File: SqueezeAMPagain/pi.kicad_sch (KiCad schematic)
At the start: 4 parts, among them J4 Raspberry_Pi_2_3

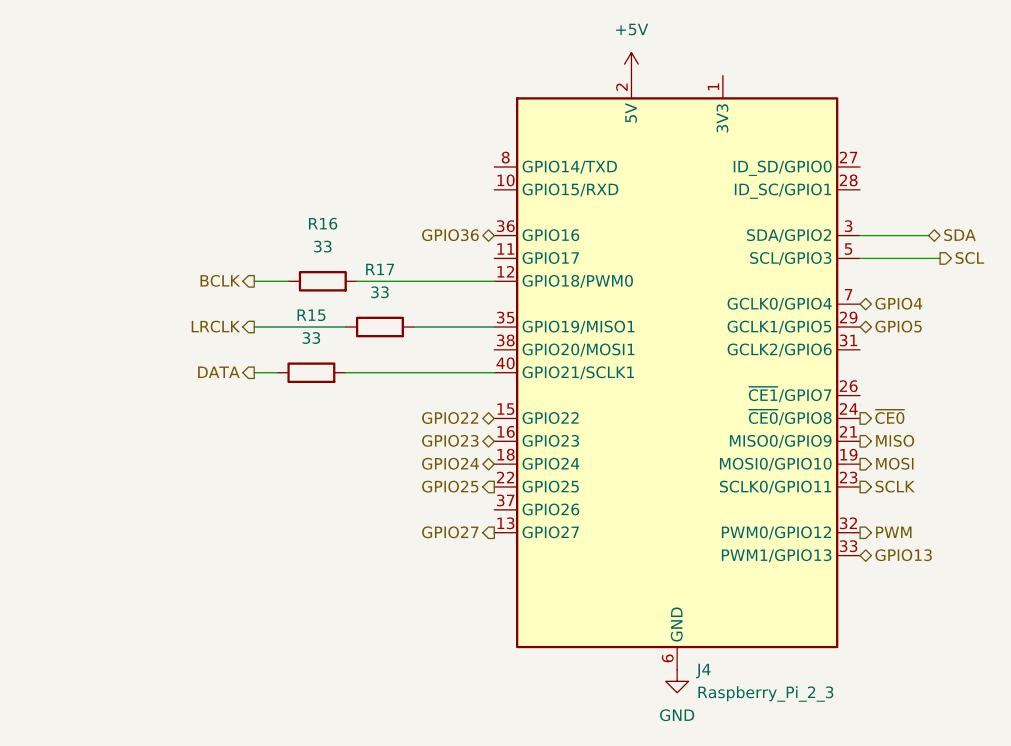
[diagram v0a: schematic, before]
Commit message: Update SqueezeAMPagain.kicad_pcb, SqueezeAMPagain.kicad_prl, SqueezeAMPagain.kicad_pro, and 7 more files
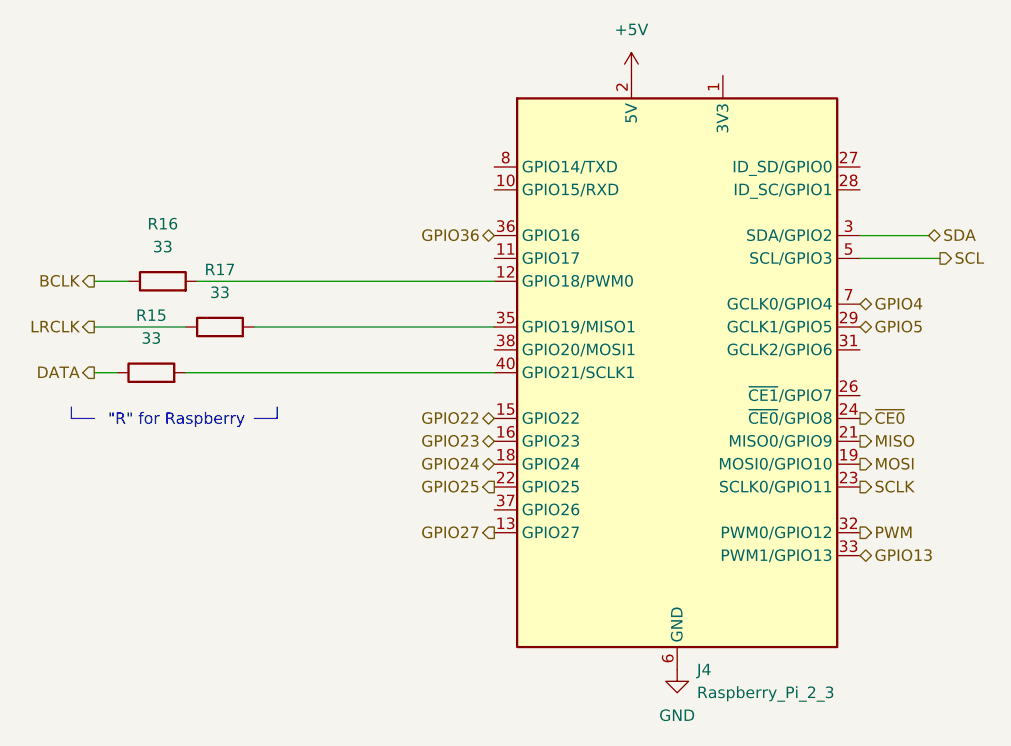
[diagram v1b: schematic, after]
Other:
- note added: ""R" for Raspberry"
- moved on the sheet: R15, R16, R17
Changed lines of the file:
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@@
 	(generator_version "8.0")
 	(paper "A4")
+	(polyline
+		(pts
+			(xy 19.05 91.44) (xy 19.05 92.71)
+		)
+		(stroke
+			(width 0)
+			(type default)
+		)
+	)
+	(polyline
+		(pts
+			(xy 41.91 91.44) (xy 41.91 92.71)
+		)
+		(stroke
+			(width 0)
+			(type default)
+		)
+	)
 	(wire
 		(pts
-			(xy 50.8 77.47) (xy 66.04 77.47)
+			(xy 33.02 77.47) (xy 66.04 77.47)
 		)
 		(stroke
@@
 		)
 	)
+	(polyline
+		(pts
+			(xy 39.37 92.71) (xy 41.91 92.71)
+		)
+		(stroke
+			(width 0)
+			(type default)
+		)
+	)
 	(wire
 		(pts
-			(xy 39.37 77.47) (xy 43.18 77.47)
+			(xy 21.59 77.47) (xy 25.4 77.47)
 		)
 		(stroke
@@
 	(wire
 		(pts
-			(xy 39.37 82.55) (xy 49.53 82.55)
+			(xy 21.59 82.55) (xy 31.75 82.55)
+		)
+		(stroke
+			(width 0)
+			(type default)
+		)
+	)
+	(polyline
+		(pts
+			(xy 19.05 92.71) (xy 21.59 92.71)
 		)
 		(stroke
@@
 	(wire
 		(pts
-			(xy 57.15 82.55) (xy 66.04 82.55)
+			(xy 39.37 82.55) (xy 66.04 82.55)
 		)
 		(stroke
@@
 	(wire
 		(pts
-			(xy 39.37 87.63) (xy 41.91 87.63)
+			(xy 21.59 87.63) (xy 24.13 87.63)
 		)
 		(stroke
@@
 	(wire
 		(pts
-			(xy 49.53 87.63) (xy 66.04 87.63)
-		)
-		(stroke
-			(width 0)
-			(type default)
+			(xy 31.75 87.63) (xy 66.04 87.63)
+		)
+		(stroke
+			(width 0)
+			(type default)
+		)
+	)
+	(text "\"R\" for Raspberry"
+		(exclude_from_sim no)
+		(at 30.734 92.964 0)
+		(effects
+			(font
+				(size 1.27 1.27)
+			)
 		)
 	)
@@
 	(hierarchical_label "LRCLK"
 		(shape output)
-		(at 39.37 82.55 180)
+		(at 21.59 82.55 180)
 		(fields_autoplaced yes)
 		(effects
@@
 	(hierarchical_label "DATA"
 		(shape output)
-		(at 39.37 87.63 180)
+		(at 21.59 87.63 180)
 		(fields_autoplaced yes)
 		(effects
@@
 	(hierarchical_label "BCLK"
 		(shape output)
-		(at 39.37 77.47 180)
+		(at 21.59 77.47 180)
 		(fields_autoplaced yes)
 		(effects
@@
 	(symbol
 		(lib_id "Device:R")
-		(at 45.72 87.63 90)
+		(at 27.94 87.63 90)
 		(unit 1)
 		(exclude_from_sim no)
@@
 		(fields_autoplaced yes)
 		(property "Reference" "R15"
-			(at 45.72 81.28 90)
+			(at 27.94 81.28 90)
 			(effects
 				(font
@@
 		)
 		(property "Value" "33"
-			(at 45.72 83.82 90)
+			(at 27.94 83.82 90)
 			(effects
 				(font
@@
 		)
 		(property "Footprint" "Resistor_SMD:R_0402_1005Metric"
-			(at 45.72 89.408 90)
+			(at 27.94 89.408 90)
 			(effects
 				(font
@@
 		)
 		(property "Datasheet" "~"
-			(at 45.72 87.63 0)
+			(at 27.94 87.63 0)
 			(effects
 				(font
@@
 		)
 		(property "Description" "Resistor"
-			(at 45.72 87.63 0)
+			(at 27.94 87.63 0)
 			(effects
 				(font
@@
 	(symbol
 		(lib_id "Device:R")
-		(at 46.99 77.47 90)
+		(at 29.21 77.47 90)
 		(unit 1)
 		(exclude_from_sim no)
@@
 		(fields_autoplaced yes)
 		(property "Reference" "R16"
-			(at 46.99 71.12 90)
+			(at 29.21 71.12 90)
 			(effects
 				(font
@@
 		)
 		(property "Value" "33"
-			(at 46.99 73.66 90)
+			(at 29.21 73.66 90)
 			(effects
 				(font
@@
 		)
 		(property "Footprint" "Resistor_SMD:R_0402_1005Metric"
-			(at 46.99 79.248 90)
+			(at 29.21 79.248 90)
 			(effects
 				(font
@@
 		)
 		(property "Datasheet" "~"
-			(at 46.99 77.47 0)
+			(at 29.21 77.47 0)
 			(effects
 				(font
@@
 		)
 		(property "Description" "Resistor"
-			(at 46.99 77.47 0)
+			(at 29.21 77.47 0)
 			(effects
 				(font
@@
 	(symbol
 		(lib_id "Device:R")
-		(at 53.34 82.55 90)
+		(at 35.56 82.55 90)
 		(unit 1)
 		(exclude_from_sim no)
@@
 		(fields_autoplaced yes)
 		(property "Reference" "R17"
-			(at 53.34 76.2 90)
+			(at 35.56 76.2 90)
 			(effects
 				(font
@@
 		)
 		(property "Value" "33"
-			(at 53.34 78.74 90)
+			(at 35.56 78.74 90)
 			(effects
 				(font
@@
 		)
 		(property "Footprint" "Resistor_SMD:R_0402_1005Metric"
-			(at 53.34 84.328 90)
+			(at 35.56 84.328 90)
 			(effects
 				(font
@@
 		)
 		(property "Datasheet" "~"
-			(at 53.34 82.55 0)
+			(at 35.56 82.55 0)
 			(effects
 				(font
@@
 		)
 		(property "Description" "Resistor"
-			(at 53.34 82.55 0)
-			(effects
-				(font
+			(at 35.56 82.55 0)
+			(effects
+				(font

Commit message: Update SqueezeAMPagain.kicad_pcb, SqueezeAMPagain.kicad_prl, SqueezeAMPagain.kicad_pro, and 11 more files
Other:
- title: (none) -> SqueezeAMP_{again}
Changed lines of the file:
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@@
 	(generator_version "8.0")
 	(paper "A4")
+	(title_block
+		(title "SqueezeAMP_{again}")
+		(date "2024-08-23")
+		(rev "1.0")
+	)
 	(polyline
 		(pts
